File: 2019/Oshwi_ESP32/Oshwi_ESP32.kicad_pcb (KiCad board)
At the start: 2 copper layers, 76.8 x 99.6 mm, 10 parts

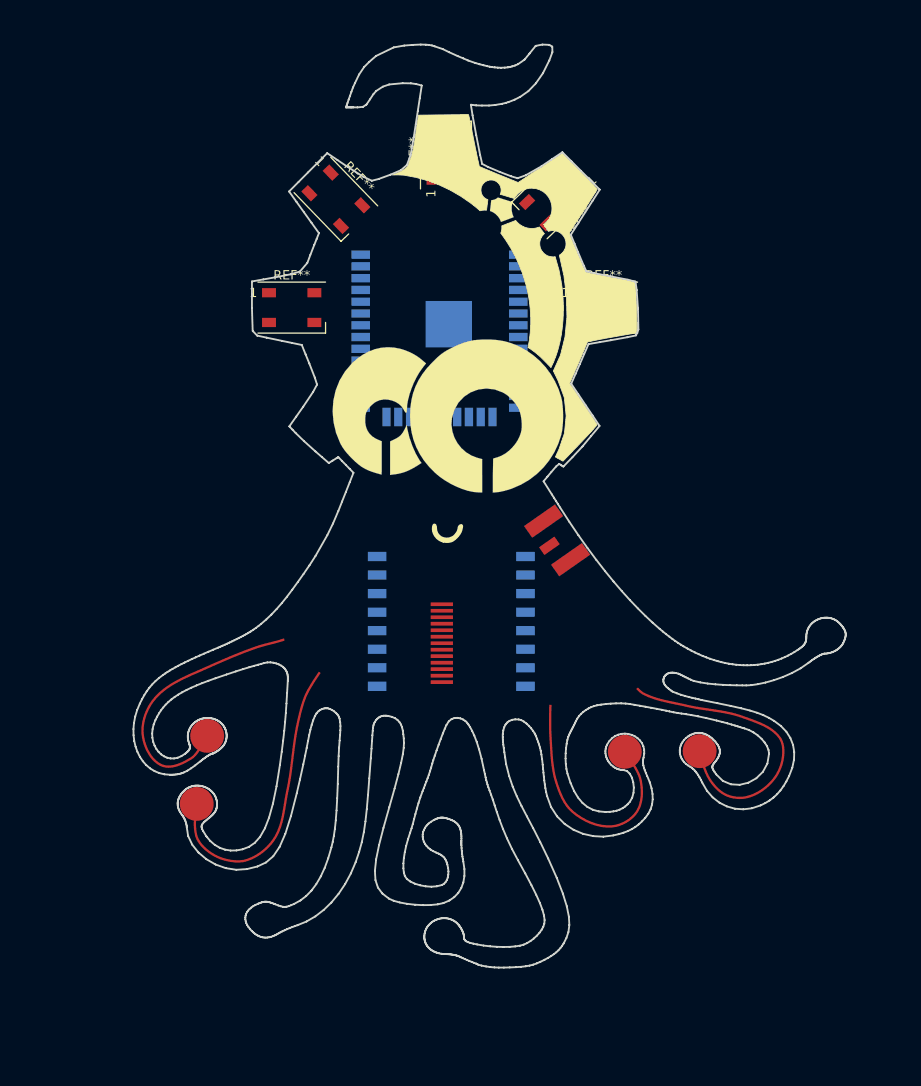
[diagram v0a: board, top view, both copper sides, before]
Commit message: Continue the Design of ESP32 Badge
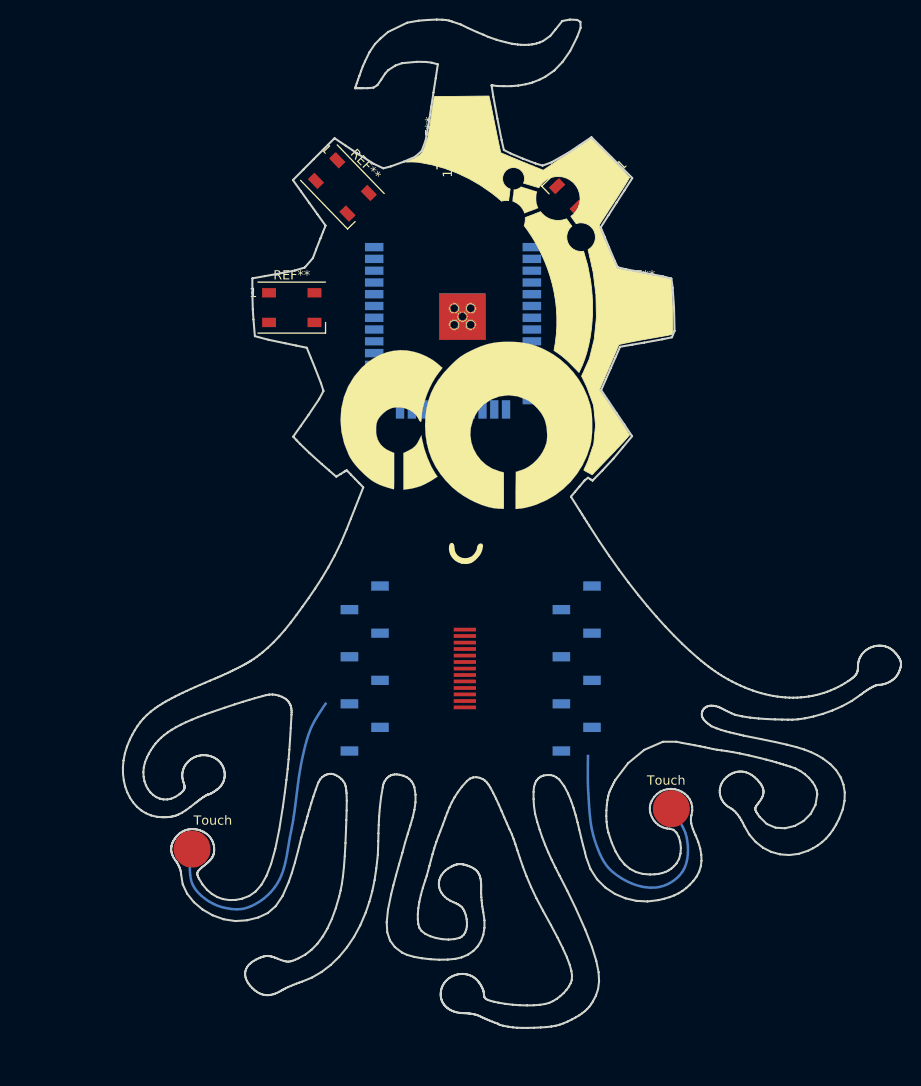
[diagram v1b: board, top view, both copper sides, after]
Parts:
- removed A2: ANT, Oshwi_ESP32:SMA_EDGELAUNCH_UFL_WeMos_Lora
- removed the REF** at (152.7, 75.9)
- removed the REF** at (154.0, 107.2)
- removed the svg2mod at (158.1, 94.7)
- added REF**: ESP32-WROOM-32, Oshwi_ESP32:ESP32-WROOM-32, B.Cu at (154.2, 75.1)
- added REF**: PinSocket_1x08_P2.54mm_Vertical_SMD_Pin1Left, Connector_PinSocket_2.54mm:PinSocket_1x08_P2.54mm_Vertical_SMD_Pin1Left, B.Cu at (144.7, 112.3)
- added REF**: PinSocket_1x08_P2.54mm_Vertical_SMD_Pin1Left, Connector_PinSocket_2.54mm:PinSocket_1x08_P2.54mm_Vertical_SMD_Pin1Left, B.Cu at (167.5, 112.3)
- added svg2mod: G***, Oshwi_ESP32:Touch_ESP32, B.Cu at (152.7, 127.1)
- added svg2mod: G***, Oshwi_ESP32:Oshwi_ESP32, F.Cu at (160.5, 96.6)
- moved REF** 3.69 mm to (155.4, 112.3)
- moved REF** 3.66 mm to (168.3, 59.7)
- moved REF** 3.56 mm to (174.0, 73.3)
- moved REF** 2.80 mm to (155.2, 54.7)
- moved REF** 1.51 mm to (142.2, 60.3)
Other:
- board size 76.8 x 99.6 mm -> 83.9 x 108.8 mm
- board text added: "Touch"

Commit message: update es8266 design
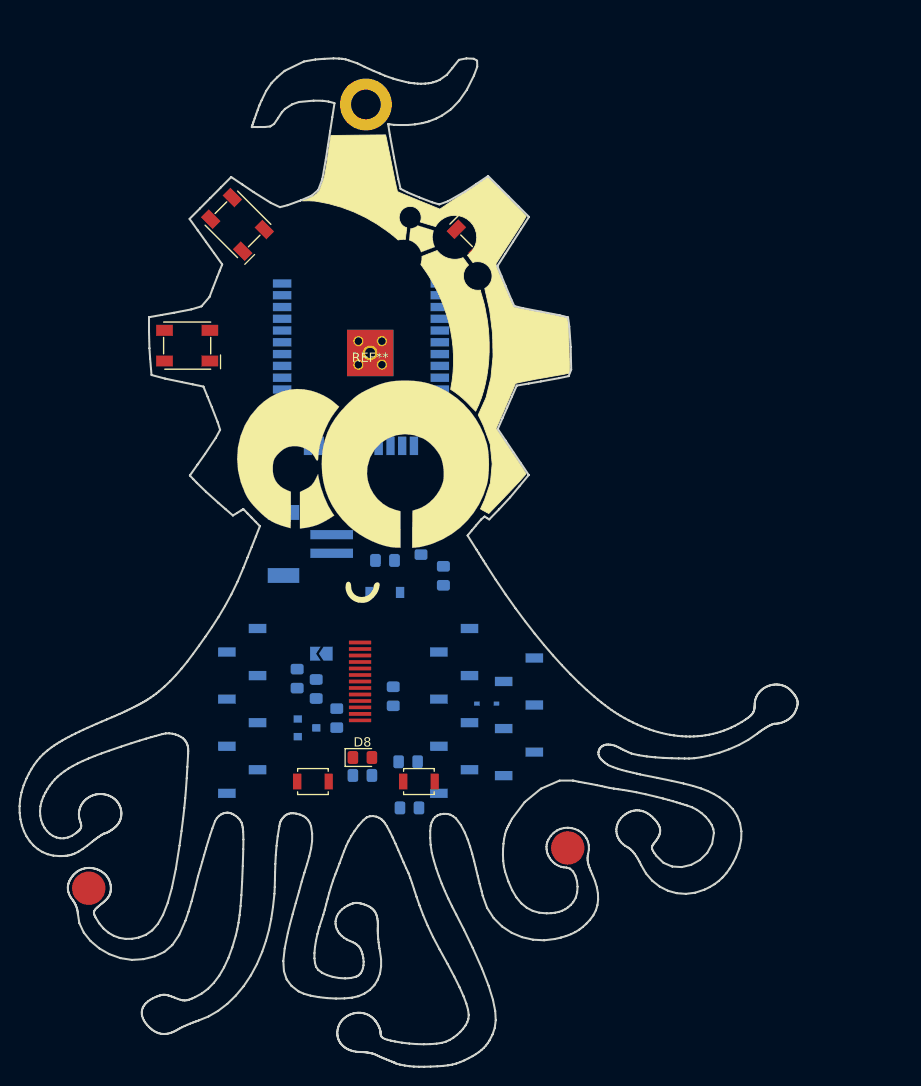
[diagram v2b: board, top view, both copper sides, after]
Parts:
- removed the REF** at (154.2, 75.1)
- removed the REF** at (144.7, 112.3)
- removed the REF** at (167.5, 112.3)
- removed the REF** at (168.3, 59.7)
- removed the REF** at (142.2, 60.3)
- removed the REF** at (155.2, 54.7)
- removed the REF** at (136.8, 73.3)
- removed the REF** at (174.0, 73.3)
- removed the REF** at (155.4, 112.3)
- removed svg2mod: G***, Oshwi_ESP32:Touch_ESP32
- removed svg2mod: G***, Oshwi_ESP32:Oshwi_ESP32
- added C1: 10uF, Capacitor_SMD:C_0805_2012Metric_Pad1.15x1.40mm_HandSolder, B.Cu at (146.8, 100.6)
- added C2: 10uF, Capacitor_SMD:C_0805_2012Metric_Pad1.15x1.40mm_HandSolder, B.Cu at (150.7, 99.0)
- added C3: 1uF, Capacitor_SMD:C_0805_2012Metric_Pad1.15x1.40mm_HandSolder, B.Cu at (153.1, 102.3)
- added C4: 1uF, Capacitor_SMD:C_0805_2012Metric_Pad1.15x1.40mm_HandSolder, B.Cu at (147.7, 115.3)
- added C5: 22nF, Capacitor_SMD:C_0805_2012Metric_Pad1.15x1.40mm_HandSolder, B.Cu at (162.7, 77.3)
- added C6: 1uF, Capacitor_SMD:C_0805_2012Metric_Pad1.15x1.40mm_HandSolder, B.Cu at (149.5, 127.3)
- added CAP1: TOUCH 1, Oshwi_ESP32:Touch_1, F.Cu at (114.9, 136.0)
- added CAP2: TOUCH 2, Oshwi_ESP32:Touch_2, F.Cu at (166.5, 131.6)
- added D1: MBR120, Diode_SMD:D_SOD-123, B.Cu at (146.8, 104.1)
- added D2: WS2812B, Oshwi_ESP32:WS2812B, F.Cu at (162.7, 77.5)
- added D3: WS2812B, Oshwi_ESP32:WS2812B, F.Cu at (157.4, 64.3)
- added D4: WS2812B, Oshwi_ESP32:WS2812B, F.Cu at (144.1, 58.4)
- added D5: WS2812B, Oshwi_ESP32:WS2812B, F.Cu at (130.9, 64.4)
- added D6: WS2812B, Oshwi_ESP32:WS2812B, F.Cu at (125.5, 77.4)
- added D7: 1N4148, Diode_SMD:D_SOD-323, B.Cu at (157.8, 116.1)
- added D8: RED, LED_SMD:LED_0805_2012Metric_Pad1.15x1.40mm_HandSolder, F.Cu at (144.4, 121.9)
- added J1: RES-A0, Connector_PinSocket_2.54mm:PinSocket_1x08_P2.54mm_Vertical_SMD_Pin1Left, B.Cu at (154.3, 116.8)
- added J2: TXD-RXD, Connector_PinSocket_2.54mm:PinSocket_1x08_P2.54mm_Vertical_SMD_Pin1Left, B.Cu at (131.4, 116.8)
- added J3: Conn_01x06, Connector_PinSocket_2.54mm:PinSocket_1x06_P2.54mm_Vertical_SMD_Pin1Left, B.Cu at (161.3, 117.5)
- added J4: JSTPH, Oshwi_ESP32:JSTPH2, B.Cu at (137.4, 98.8)
- added JP1: Jumper_NO, Jumper:SolderJumper-2_P1.3mm_Open_TrianglePad1.0x1.5mm, B.Cu at (140.0, 110.7)
- added Q1: S8050, Package_TO_SOT_SMD:SOT-23, B.Cu at (138.4, 118.7)
- added R1: 10ohm, Resistor_SMD:R_0805_2012Metric_Pad1.15x1.40mm_HandSolder, B.Cu at (141.6, 117.6)
- added R2: 1k, Resistor_SMD:R_0805_2012Metric_Pad1.15x1.40mm_HandSolder, B.Cu at (137.4, 113.4)
- added R3: 10k, Resistor_SMD:R_0805_2012Metric_Pad1.15x1.40mm_HandSolder, B.Cu at (139.4, 114.5)
- added R4: 10K, Resistor_SMD:R_0805_2012Metric_Pad1.15x1.40mm_HandSolder, B.Cu at (149.3, 122.3)
- added R5: 1K, Resistor_SMD:R_0805_2012Metric_Pad1.15x1.40mm_HandSolder, B.Cu at (144.4, 123.8)
- added REF**: Thermal_ESP32, Oshwi_ESP32:Thermal_ESP32, F.Cu at (145.2, 78.2)
- added REF**: MountingHole_3.2mm_M3_DIN965_Pad, Oshwi_ESP32:MountingHole_3.2mm_M3_DIN965_Pad, F.Cu at (144.8, 51.4)
- added SW1: SW_Push, Oshwi_ESP32:SW_SPST_B3U-1000P, F.Cu at (139.1, 124.5)
- added SW2: SW_Push, Oshwi_ESP32:SW_SPST_B3U-1000P, F.Cu at (150.5, 124.5)
- added U1: AP2112-3.3, Package_TO_SOT_SMD:SOT-23-5, B.Cu at (146.8, 97.1)
- added U2: TFT_0.9680*160, Display:TFT_0.96_SPI, F.Cu at (144.1, 113.7)
- added U3: ESP32-WROOM-32D, RF_Module:ESP32-WROOM-32, B.Cu at (144.2, 79.0)
- added U4: Oshwi_Edge_Cut, Oshwi_ESP32:Oshwi_ESP32, F.Cu at (144.3, 101.5)
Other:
- outline, holes or cut-outs redrawn
- net class Default: trace_width 0.1524 -> 0.25; via_dia 0.508 -> 0.6858; via_drill 0.254 -> 0.3302
- net class Power added: clearance 0.1524, trace_width 0.6096, via_dia 0.6858, via_drill 0.3302
- rule pad_to_mask_clearance: 0.0508 -> 0.0762
- rule via_min_drill: 0.254 -> 0.3302
- rule via_min_size: 0.508 -> 0.6858
- board text removed: "Touch"
